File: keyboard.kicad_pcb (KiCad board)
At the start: 2 copper layers, 168.3 x 124.5 mm, 68 parts, among them J1 Conn_01x06_Socket, J3 Conn_01x02_Socket, SW1 SW_Push, SW10 SW_Push, SW11 SW_Push, SW12 SW_Push, SW13 SW_Push, SW14 SW_Push, SW15 SW_Push, SW16 SW_Push, SW17 SW_Push, SW18 SW_Push, SW19 SW_Push, SW2 SW_Push, SW20 SW_Push, SW21 SW_Push, SW22 SW_Push, SW23 SW_Push, SW24 SW_Push, SW25 SW_Push, SW26 SW_Push, SW27 SW_Push, SW28 SW_Push, SW29 SW_Push, SW3 SW_Push, SW30 SW_Push, SW4 SW_Push, SW5 SW_Push, SW6 SW_Push, SW7 SW_Push, SW8 SW_Push, SW9 SW_Push, U1 rp2040-zero

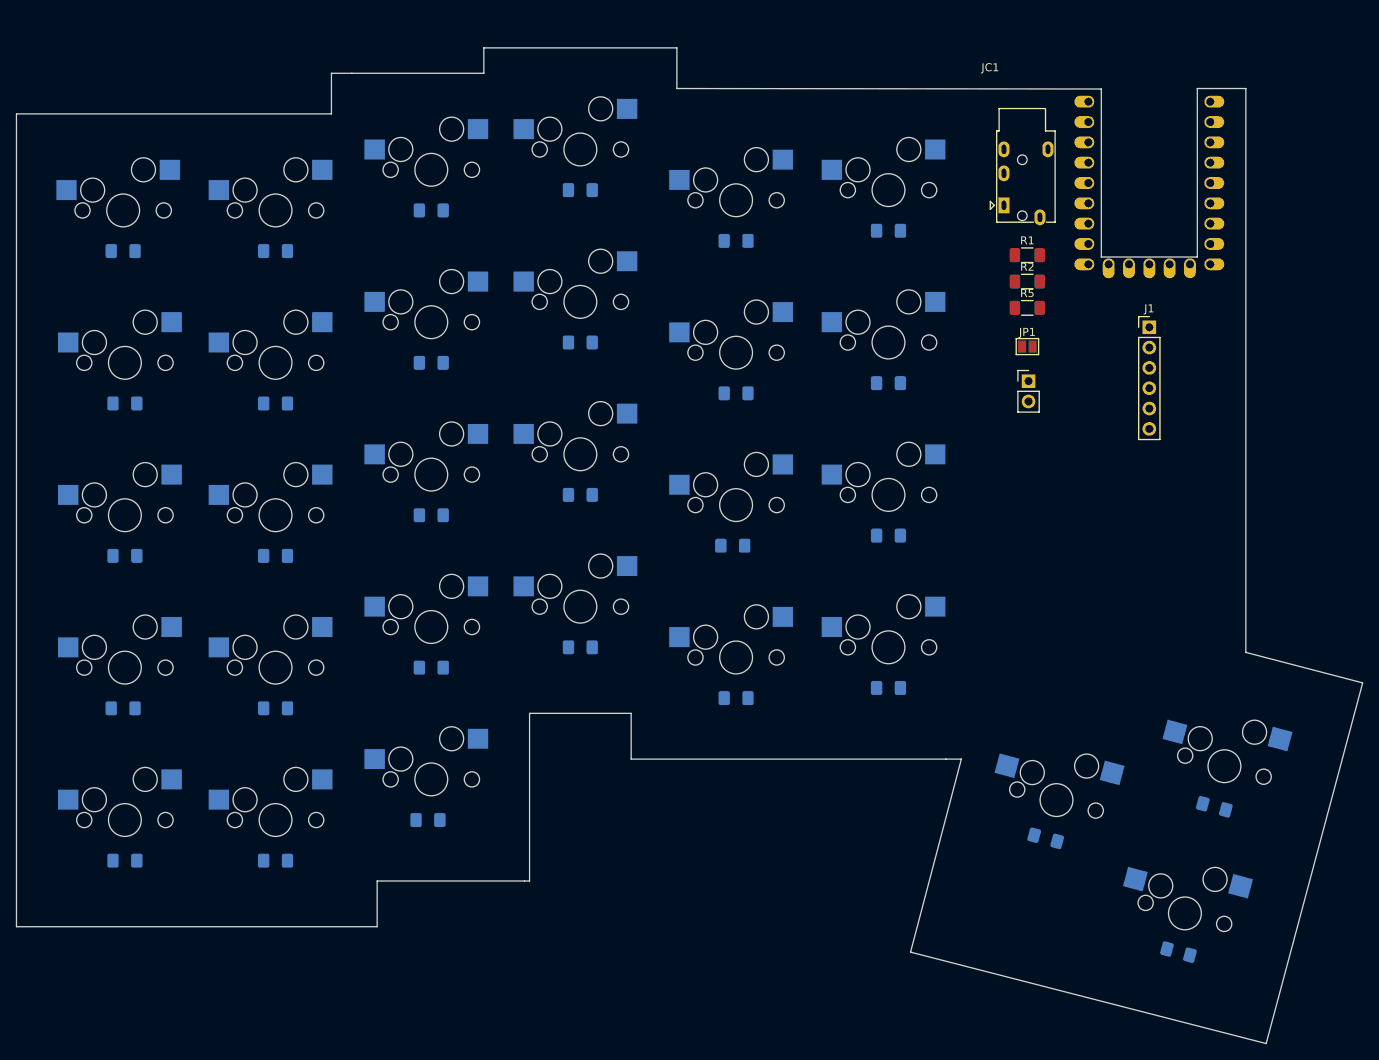
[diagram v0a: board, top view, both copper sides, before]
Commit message: 一旦保存2
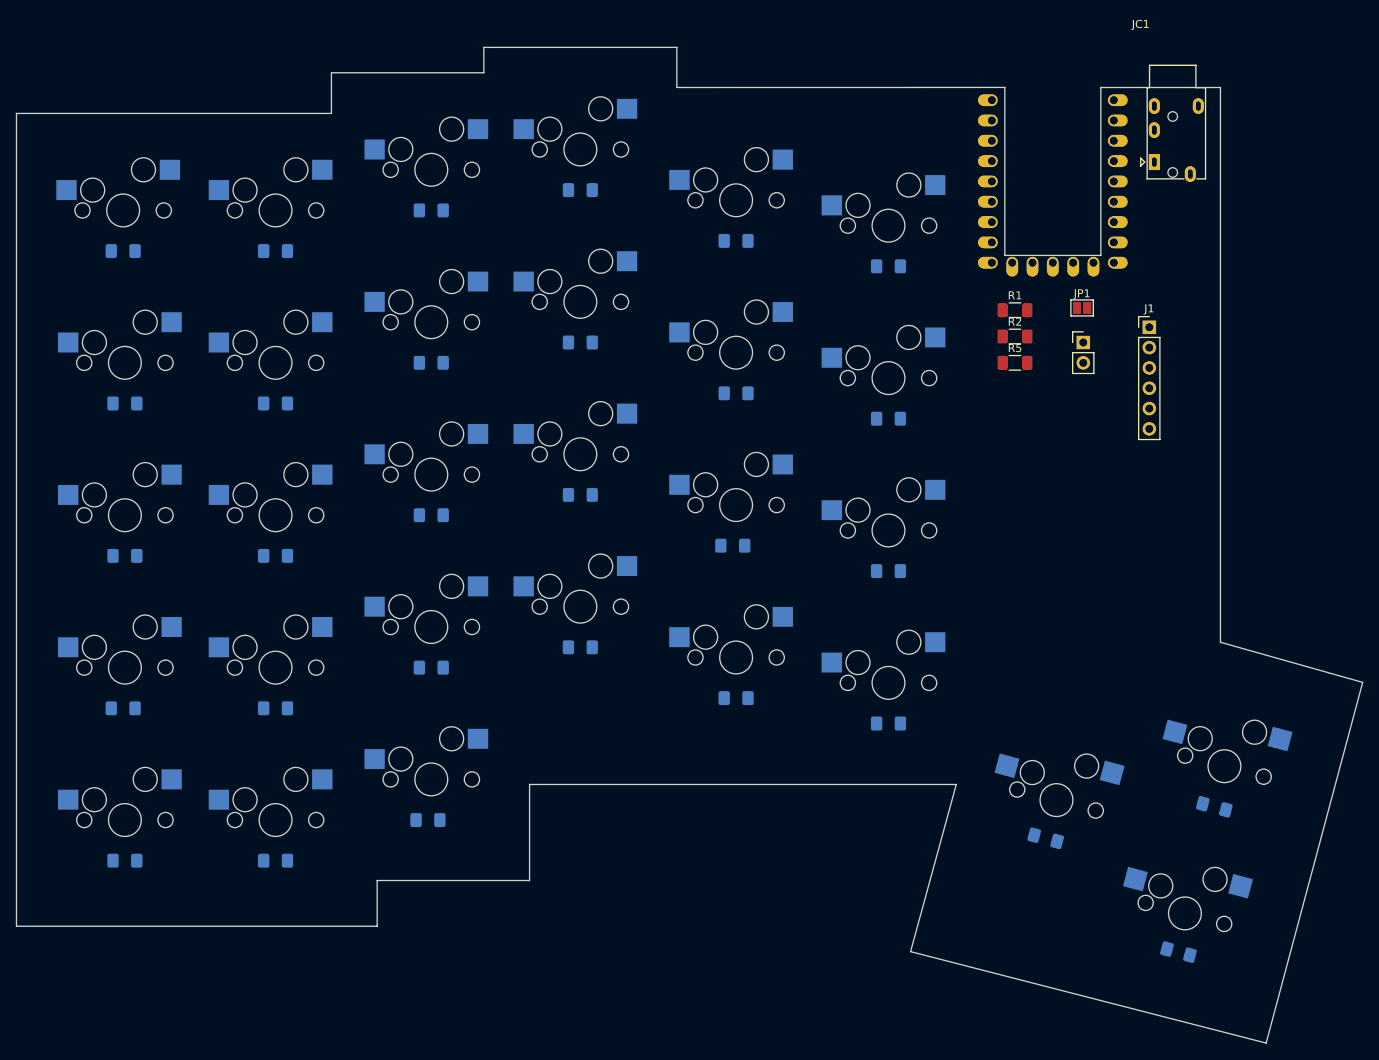
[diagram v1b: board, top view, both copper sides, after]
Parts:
- moved JC1 19.6 mm to (205.1, 51.7)
- moved U1 12.1 mm to (192.4, 54.2)
- moved JP1 8.37 mm to (196.1, 70.0)
- moved J3 8.37 mm to (196.2, 74.3)
- moved R2 7.04 mm to (187.7, 73.5)
- moved R1 7.04 mm to (187.7, 70.3)
- moved R5 7.04 mm to (187.7, 76.8)
- moved D23 4.45 mm to (171.9, 102.9)
- moved D24 4.45 mm to (171.9, 121.9)
- moved SW23 4.45 mm to (171.9, 97.8)
- moved SW24 4.45 mm to (171.9, 116.8)
- moved SW21 4.45 mm to (171.9, 59.7)
- moved D21 4.44 mm to (171.9, 64.8)
- moved D22 4.44 mm to (171.9, 83.8)
- moved SW22 4.44 mm to (171.9, 78.7)
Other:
- outline, holes or cut-outs redrawn

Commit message: pcb大体並べたので一旦保存
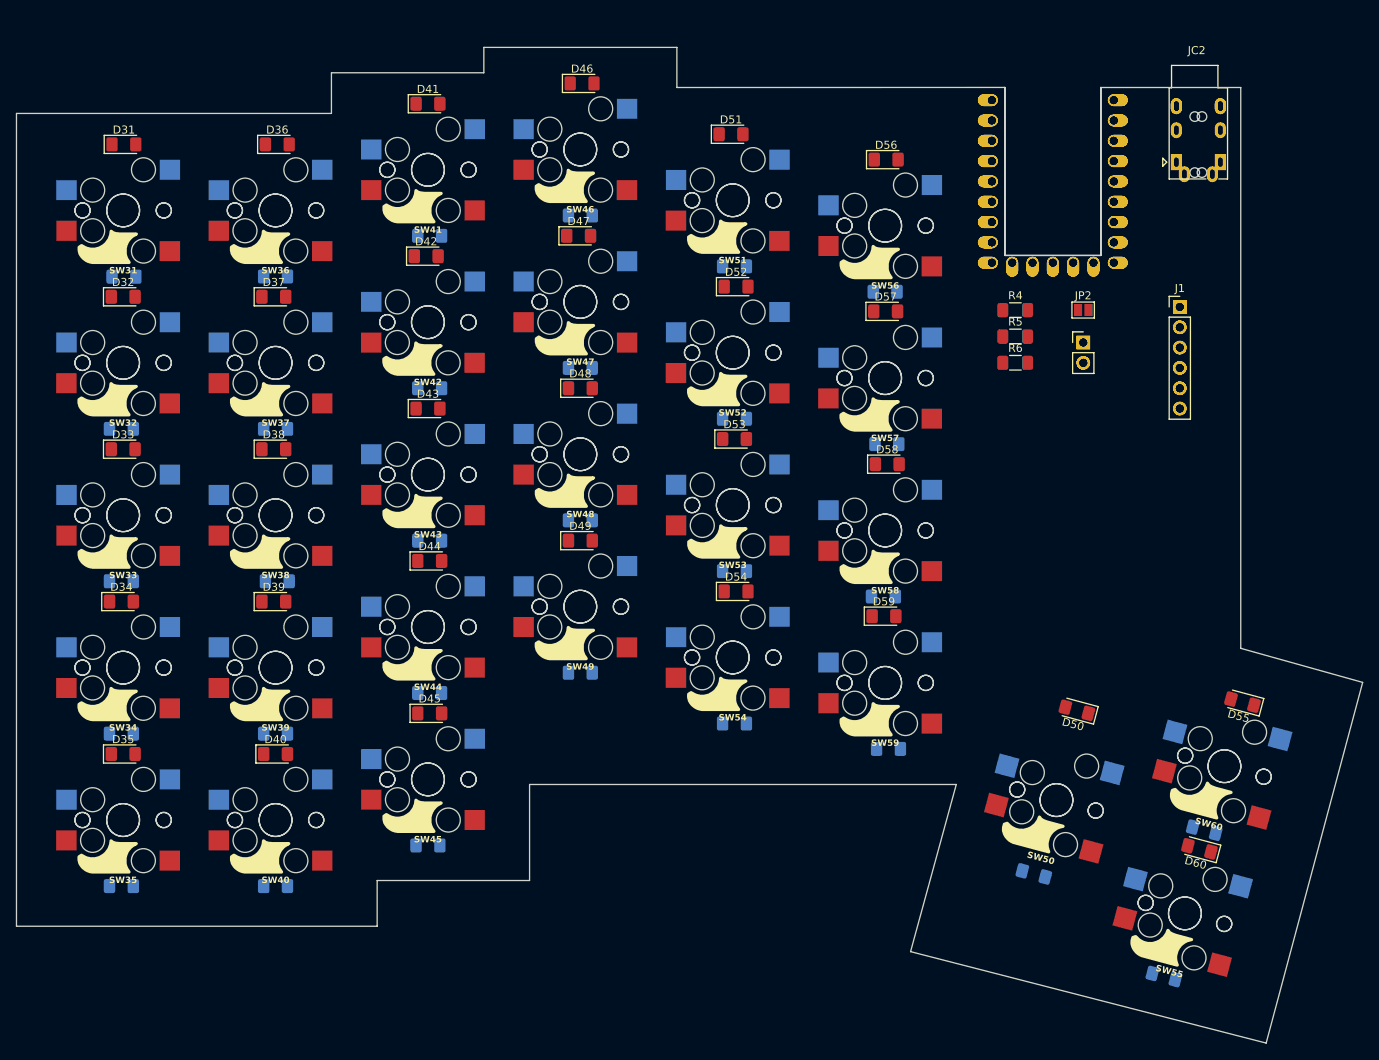
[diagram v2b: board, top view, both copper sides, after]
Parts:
- added D31: D, Diode_SMD:D_1206_3216Metric_Pad1.42x1.75mm_HandSolder, F.Cu at (76.3, 49.5)
- added D32: D, Diode_SMD:D_1206_3216Metric_Pad1.42x1.75mm_HandSolder, F.Cu at (76.2, 68.6)
- added D33: D, Diode_SMD:D_1206_3216Metric_Pad1.42x1.75mm_HandSolder, F.Cu at (76.2, 87.6)
- added D34: D, Diode_SMD:D_1206_3216Metric_Pad1.42x1.75mm_HandSolder, F.Cu at (76.0, 106.7)
- added D35: D, Diode_SMD:D_1206_3216Metric_Pad1.42x1.75mm_HandSolder, F.Cu at (76.2, 125.7)
- added D36: D, Diode_SMD:D_1206_3216Metric_Pad1.42x1.75mm_HandSolder, F.Cu at (95.5, 49.5)
- added D37: D, Diode_SMD:D_1206_3216Metric_Pad1.42x1.75mm_HandSolder, F.Cu at (95.0, 68.6)
- added D38: D, Diode_SMD:D_1206_3216Metric_Pad1.42x1.75mm_HandSolder, F.Cu at (95.0, 87.6)
- added D39: D, Diode_SMD:D_1206_3216Metric_Pad1.42x1.75mm_HandSolder, F.Cu at (95.0, 106.7)
- added D40: D, Diode_SMD:D_1206_3216Metric_Pad1.42x1.75mm_HandSolder, F.Cu at (95.2, 125.7)
- added D41: D, Diode_SMD:D_1206_3216Metric_Pad1.42x1.75mm_HandSolder, F.Cu at (114.3, 44.5)
- added D42: D, Diode_SMD:D_1206_3216Metric_Pad1.42x1.75mm_HandSolder, F.Cu at (114.1, 63.5)
- added D43: D, Diode_SMD:D_1206_3216Metric_Pad1.42x1.75mm_HandSolder, F.Cu at (114.3, 82.5)
- added D44: D, Diode_SMD:D_1206_3216Metric_Pad1.42x1.75mm_HandSolder, F.Cu at (114.5, 101.6)
- added D45: D, Diode_SMD:D_1206_3216Metric_Pad1.42x1.75mm_HandSolder, F.Cu at (114.5, 120.7)
- added D46: D, Diode_SMD:D_1206_3216Metric_Pad1.42x1.75mm_HandSolder, F.Cu at (133.6, 41.9)
- added D47: D, Diode_SMD:D_1206_3216Metric_Pad1.42x1.75mm_HandSolder, F.Cu at (133.1, 61.0)
- added D48: D, Diode_SMD:D_1206_3216Metric_Pad1.42x1.75mm_HandSolder, F.Cu at (133.3, 80.0)
- added D49: D, Diode_SMD:D_1206_3216Metric_Pad1.42x1.75mm_HandSolder, F.Cu at (133.3, 99.1)
- added D50: D, Diode_SMD:D_1206_3216Metric_Pad1.42x1.75mm_HandSolder, F.Cu at (195.4, 120.3)
- added D51: D, Diode_SMD:D_1206_3216Metric_Pad1.42x1.75mm_HandSolder, F.Cu at (152.2, 48.3)
- added D52: D, Diode_SMD:D_1206_3216Metric_Pad1.42x1.75mm_HandSolder, F.Cu at (152.8, 67.3)
- added D53: D, Diode_SMD:D_1206_3216Metric_Pad1.42x1.75mm_HandSolder, F.Cu at (152.6, 86.4)
- added D54: D, Diode_SMD:D_1206_3216Metric_Pad1.42x1.75mm_HandSolder, F.Cu at (152.8, 105.4)
- added D55: D, Diode_SMD:D_1206_3216Metric_Pad1.42x1.75mm_HandSolder, F.Cu at (216.1, 119.2)
- added D56: D, Diode_SMD:D_1206_3216Metric_Pad1.42x1.75mm_HandSolder, F.Cu at (171.6, 51.4)
- added D57: D, Diode_SMD:D_1206_3216Metric_Pad1.42x1.75mm_HandSolder, F.Cu at (171.5, 70.4)
- added D58: D, Diode_SMD:D_1206_3216Metric_Pad1.42x1.75mm_HandSolder, F.Cu at (171.7, 89.5)
- added D59: D, Diode_SMD:D_1206_3216Metric_Pad1.42x1.75mm_HandSolder, F.Cu at (171.3, 108.5)
- added D60: D, Diode_SMD:D_1206_3216Metric_Pad1.42x1.75mm_HandSolder, F.Cu at (210.7, 137.6)
- added J2: Conn_01x02_Socket, Connector_PinHeader_2.54mm:PinHeader_1x02_P2.54mm_Vertical, B.Cu at (196.2, 74.3)
- added J4: Conn_01x06_Socket, Connector_PinHeader_2.54mm:PinHeader_1x06_P2.54mm_Vertical, B.Cu at (208.3, 69.8)
- added JC2: AudioJack4, Connector_Audio:Jack_3.5mm_PJ320E_Horizontal, F.Cu at (207.8, 51.8)
- added JP2: Jumper_2_Open, Jumper:SolderJumper-2_P1.3mm_Open_Pad1.0x1.5mm, F.Cu at (196.2, 70.2)
- added R4: R, Resistor_SMD:R_1206_3216Metric_Pad1.30x1.75mm_HandSolder, F.Cu at (187.7, 70.2)
- added R5: R, Resistor_SMD:R_1206_3216Metric_Pad1.30x1.75mm_HandSolder, F.Cu at (187.7, 73.5)
- added R6: R, Resistor_SMD:R_1206_3216Metric_Pad1.30x1.75mm_HandSolder, F.Cu at (187.7, 76.8)
- added SW31: SW_Push, kbd:keyswitch_cherrymx_hotswap_1u, F.Cu at (76.2, 57.8)
- added SW32: SW_Push, kbd:keyswitch_cherrymx_hotswap_1u, F.Cu at (76.2, 76.8)
- added SW33: SW_Push, kbd:keyswitch_cherrymx_hotswap_1u, F.Cu at (76.2, 95.9)
- added SW34: SW_Push, kbd:keyswitch_cherrymx_hotswap_1u, F.Cu at (76.2, 114.9)
- added SW35: SW_Push, kbd:keyswitch_cherrymx_hotswap_1u, F.Cu at (76.2, 134.0)
- added SW36: SW_Push, kbd:keyswitch_cherrymx_hotswap_1u, F.Cu at (95.2, 57.8)
- added SW37: SW_Push, kbd:keyswitch_cherrymx_hotswap_1u, F.Cu at (95.2, 76.8)
- added SW38: SW_Push, kbd:keyswitch_cherrymx_hotswap_1u, F.Cu at (95.2, 95.9)
- added SW39: SW_Push, kbd:keyswitch_cherrymx_hotswap_1u, F.Cu at (95.2, 114.9)
- added SW40: SW_Push, kbd:keyswitch_cherrymx_hotswap_1u, F.Cu at (95.2, 134.0)
- added SW41: SW_Push, kbd:keyswitch_cherrymx_hotswap_1u, F.Cu at (114.3, 52.7)
- added SW42: SW_Push, kbd:keyswitch_cherrymx_hotswap_1u, F.Cu at (114.3, 71.8)
- added SW43: SW_Push, kbd:keyswitch_cherrymx_hotswap_1u, F.Cu at (114.3, 90.8)
- added SW44: SW_Push, kbd:keyswitch_cherrymx_hotswap_1u, F.Cu at (114.3, 109.9)
- added SW45: SW_Push, kbd:keyswitch_cherrymx_hotswap_1u, F.Cu at (114.3, 128.9)
- added SW46: SW_Push, kbd:keyswitch_cherrymx_hotswap_1u, F.Cu at (133.3, 50.2)
- added SW47: SW_Push, kbd:keyswitch_cherrymx_hotswap_1u, F.Cu at (133.3, 69.2)
- added SW48: SW_Push, kbd:keyswitch_cherrymx_hotswap_1u, F.Cu at (133.3, 88.3)
- added SW49: SW_Push, kbd:keyswitch_cherrymx_hotswap_1u, F.Cu at (133.3, 107.3)
- added SW50: SW_Push, kbd:keyswitch_cherrymx_hotswap_2u_vertical, F.Cu at (192.9, 131.5)
- added SW51: SW_Push, kbd:keyswitch_cherrymx_hotswap_1u, F.Cu at (152.4, 56.5)
- added SW52: SW_Push, kbd:keyswitch_cherrymx_hotswap_1u, F.Cu at (152.4, 75.6)
- added SW53: SW_Push, kbd:keyswitch_cherrymx_hotswap_1u, F.Cu at (152.4, 94.6)
- added SW54: SW_Push, kbd:keyswitch_cherrymx_hotswap_1u, F.Cu at (152.4, 113.7)
- added SW55: SW_Push, kbd:keyswitch_cherrymx_hotswap_1u, F.Cu at (208.9, 145.7)
- added SW56: SW_Push, kbd:keyswitch_cherrymx_hotswap_1u, F.Cu at (171.4, 59.7)
- added SW57: SW_Push, kbd:keyswitch_cherrymx_hotswap_1u, F.Cu at (171.4, 78.7)
- added SW58: SW_Push, kbd:keyswitch_cherrymx_hotswap_1u, F.Cu at (171.4, 97.8)
- added SW59: SW_Push, kbd:keyswitch_cherrymx_hotswap_1u, F.Cu at (171.4, 116.8)
- added SW60: SW_Push, kbd:keyswitch_cherrymx_hotswap_1u, F.Cu at (213.9, 127.3)
- added U2: rp2040-zero, mcu:rp2040-zero-tht, F.Cu at (192.4, 54.2)
- JC1, JP1, R1, R2: moved to B.Cu
- R3: renamed from R5; moved to B.Cu
- moved D29 20.1 mm to (171.9, 125.1)
- moved D27 19.9 mm to (171.7, 87.0)
- moved D28 19.9 mm to (171.2, 106.0)
- moved SW23 19.7 mm to (152.4, 94.6)
- moved SW21 19.7 mm to (152.4, 56.5)
- moved SW22 19.7 mm to (152.4, 75.6)
- moved SW24 19.7 mm to (152.4, 113.7)
- moved D26 19.7 mm to (171.4, 67.9)
- moved D21 19.2 mm to (152.6, 64.8)
- moved D22 19.2 mm to (152.6, 83.8)
- moved D23 19.2 mm to (152.6, 102.9)
- moved D24 19.2 mm to (152.6, 121.9)
- moved SW28 18.9 mm to (171.4, 97.8)
- moved SW26 18.9 mm to (171.4, 59.7)
- moved SW27 18.9 mm to (171.4, 78.7)
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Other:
- outline, holes or cut-outs redrawn
